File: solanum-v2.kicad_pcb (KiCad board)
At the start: 2 copper layers, 143.6 x 93.8 mm, 29 parts, among them J1 Battery_Cell, J2 AudioJack4, SW1 SW_Push_45deg, SW10 SW_Push_45deg, SW11 SW_Push_45deg, SW12 SW_Push_45deg, SW13 SW_Push_45deg, SW14 SW_Push_45deg, SW15 SW_Push_45deg, SW16 SW_Push_45deg, SW17 SW_Push_45deg, SW18 SW_SPDT, SW2 SW_Push_45deg, SW3 SW_Push_45deg, SW4 SW_Push_45deg, SW5 SW_Push_45deg, SW6 SW_Push_45deg, SW7 SW_Push_45deg, SW8 SW_Push_45deg, SW9 SW_Push_45deg, U1 ProMicro, X1 Tenting puck

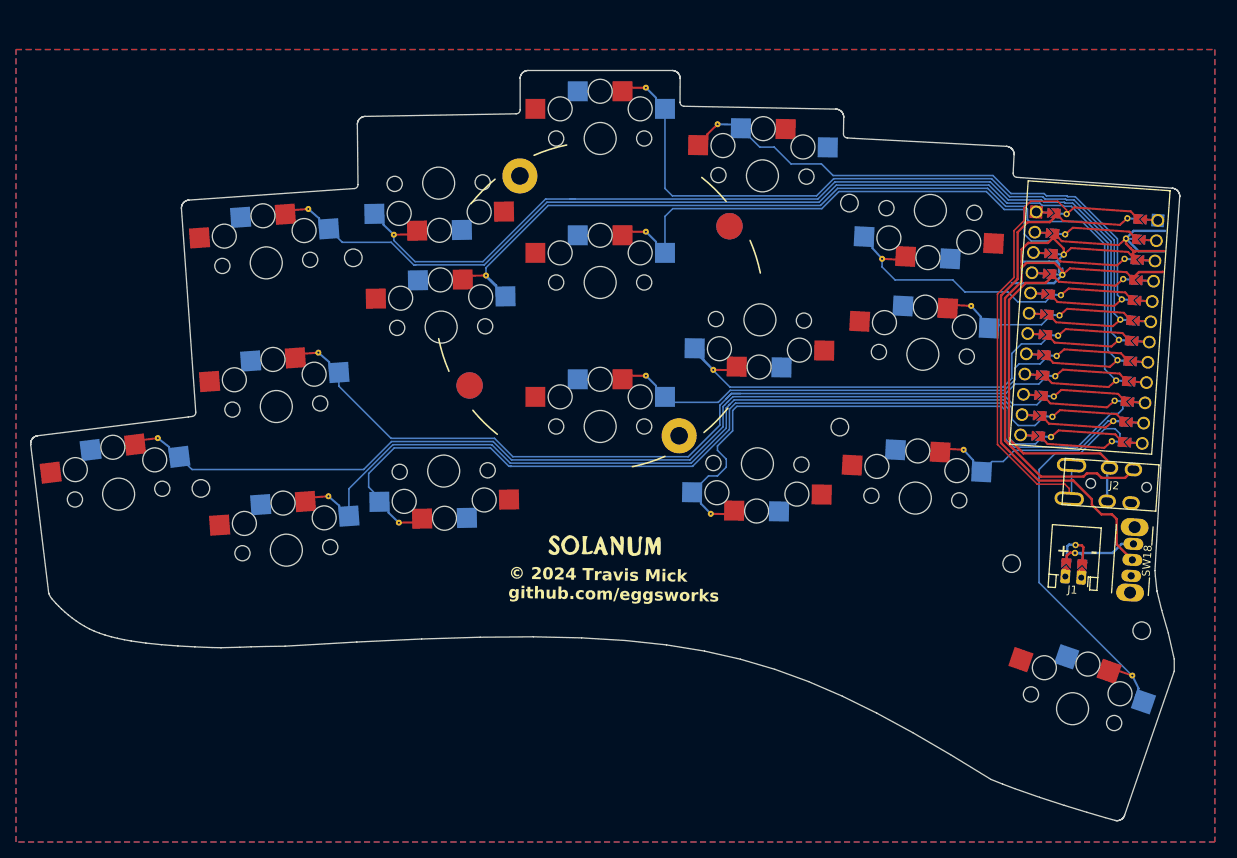
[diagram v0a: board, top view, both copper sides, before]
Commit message: progress on v2 pcb
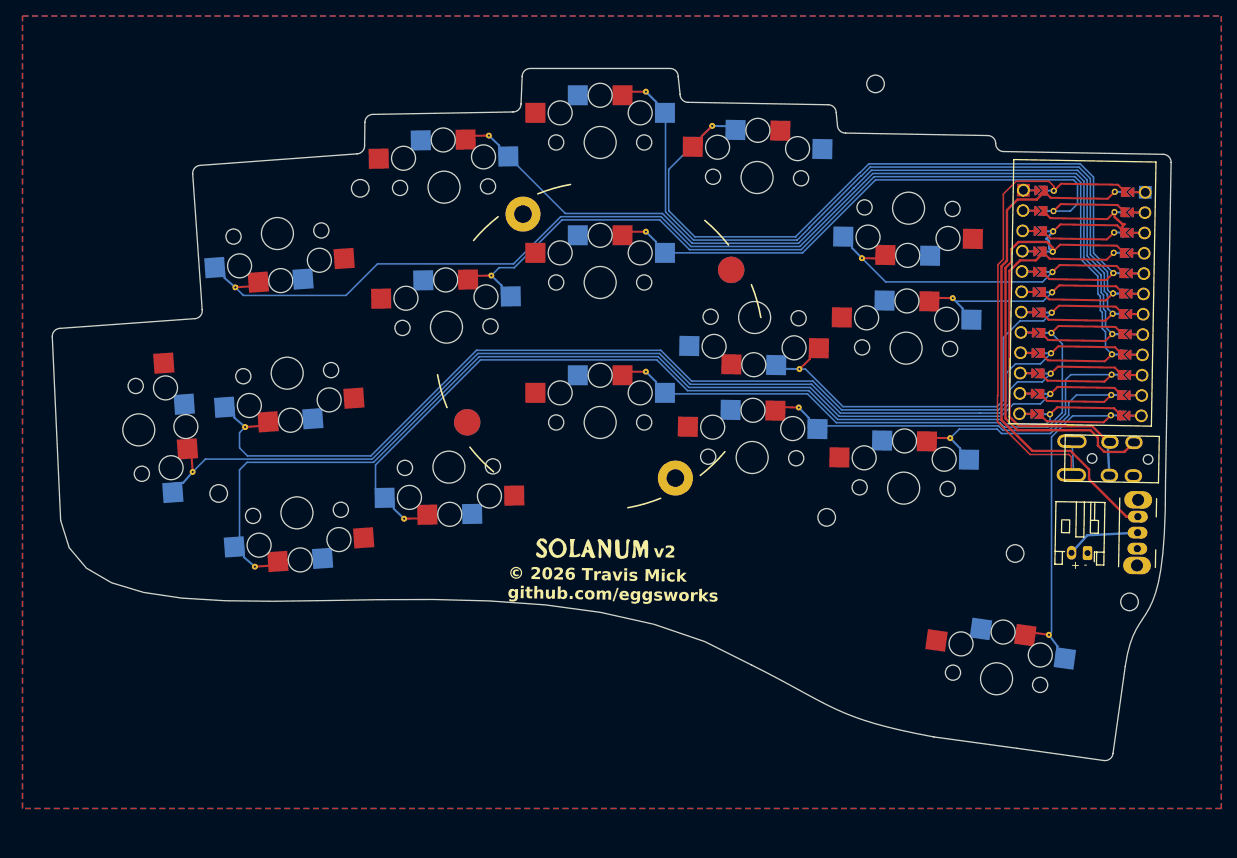
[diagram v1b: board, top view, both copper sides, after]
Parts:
- J1: footprint Library:JST_PH_S2B-PH-K_1x02_P2.00mm_Horizontal -> Connector_JST:JST_PH_S2B-PH-K_1x02_P2.00mm_Horizontal
- SW9: moved to B.Cu
- moved H4 15.3 mm to (181.1, 59.8)
- moved H6 11.4 mm to (175.0, 114.0)
- moved SW16 10.2 mm to (196.2, 134.2), turned to -8 degrees
- moved H5 8.73 mm to (116.7, 72.9)
- moved SW17 8.42 mm to (89.0, 103.1), turned to -86 degrees
- moved X1 5.03 mm to (146.6, 92.6), turned to 30 degrees
- moved SW11 4.85 mm to (108.8, 113.4), turned to -176 degrees
- moved SW6 4.38 mm to (107.6, 96.0), turned to -176 degrees
- moved SW1 3.92 mm to (106.4, 78.5), turned to -176 degrees
- moved H1 3.91 mm to (212.9, 124.6), turned to -1 degrees
- moved J2 3.57 mm to (216.7, 106.8), turned to -91 degrees
- moved SW18 3.48 mm to (213.8, 117.9), turned to 89 degrees
- moved U1 3.20 mm to (207.0, 87.2), turned to -91 degrees
- moved J1 3.17 mm to (207.6, 118.5), turned to 179 degrees
- moved SW5 2.74 mm to (185.2, 75.4), turned to 179 degrees
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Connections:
- SW18 pad 2: RAW -> Net-(J1-Pin_2)
- SW18 pad 3: Net-(J1-Pin_2) -> RAW
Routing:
- net GND: track 95.8 -> 53.2 mm
- net SW14: track 70.0 -> 42.0 mm
- net SW4: track 60.6 -> 84.8 mm
- net SW11: track 101.2 -> 121.3 mm
- net SW6: track 101.7 -> 118.3 mm
- net SW1: track 122.6 -> 137.8 mm
- net SW2: track 113.0 -> 100.2 mm
- net SW16: track 45.5 -> 33.3 mm
- net SW13: track 51.5 -> 62.5 mm
- net SW3: track 81.6 -> 91.5 mm
- net SW9: track 51.2 -> 43.0 mm
- net SW10: track 8.48 -> 13.0 mm
- net SW15: track 20.4 -> 23.7 mm
- net SW7: track 108.6 -> 105.3 mm
- net RAW: track 58.0 -> 55.2 mm
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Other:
- board size 143.6 x 93.8 mm -> 139.9 x 86.5 mm
- board text added: "1"
- board text added: "3"
- board text added: "v2"
- board text added: "© 2026 Travis Mick github.com/eggsworks"
- board text removed: "© 2024 Travis Mick github.com/eggsworks"
